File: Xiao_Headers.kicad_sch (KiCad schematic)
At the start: 22 parts, among them J1 Barrel_Jack, P1 USB_C_Plug_USB2.0, SW1 SW_Push, U1 SHT4x, U2 ESP32-C3-WROOM-02, U3 TSL25911FN, U5 LT1963AxST-3.3

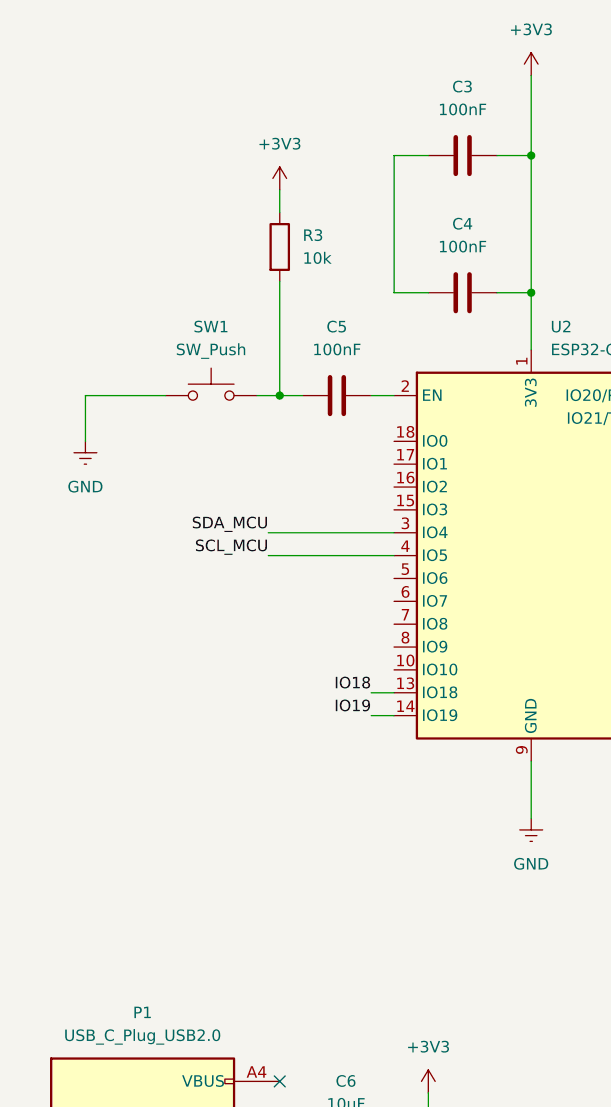
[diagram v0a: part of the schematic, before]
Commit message: Finalize MCU Minsys
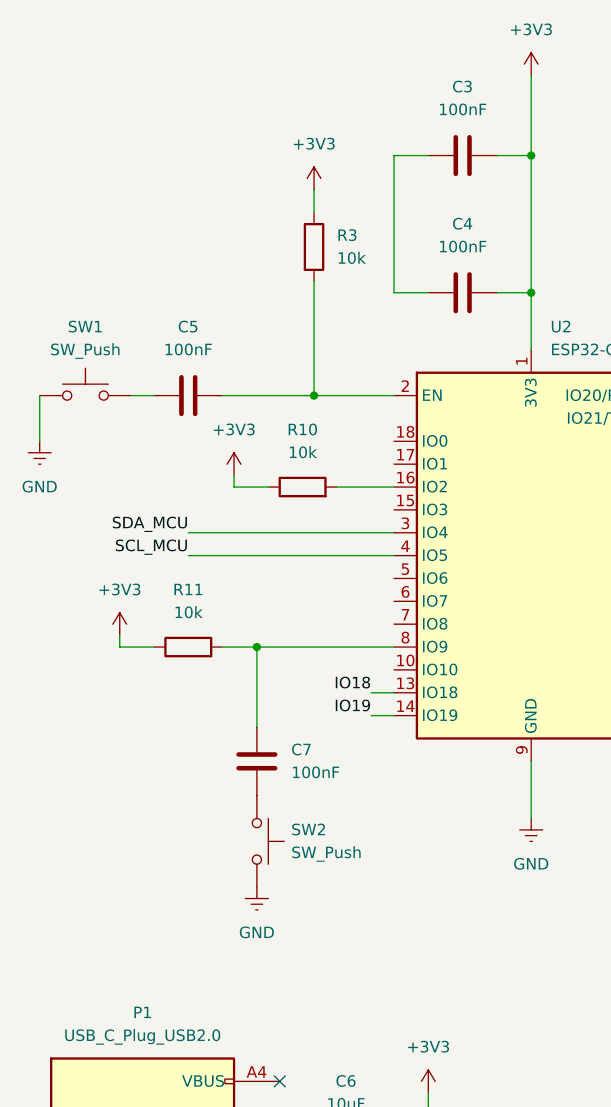
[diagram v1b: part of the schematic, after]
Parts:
- added C7: 100nF, symbol Device:C
- added R10, R11: 10k, symbol Device:R
- added SW2: SW_Push, symbol Switch:SW_Push
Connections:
- net +3V3: now also R10.1, R11.1
- net GND: now also SW2.2
- net at C5.1, SW1.2: no longer R3.2
- net at U2.16 (IO2): now also R10.2
- net at C5.2, U2.2 (EN): now also R3.2
- net at U2.8 (IO9): now also C7.2, R11.2
- new net: C7.1, SW2.1
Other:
- moved on the sheet: R3, SW1
